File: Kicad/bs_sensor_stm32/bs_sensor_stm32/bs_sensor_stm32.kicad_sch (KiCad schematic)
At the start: 4 parts, among them U1 NRF24L01_Breakout

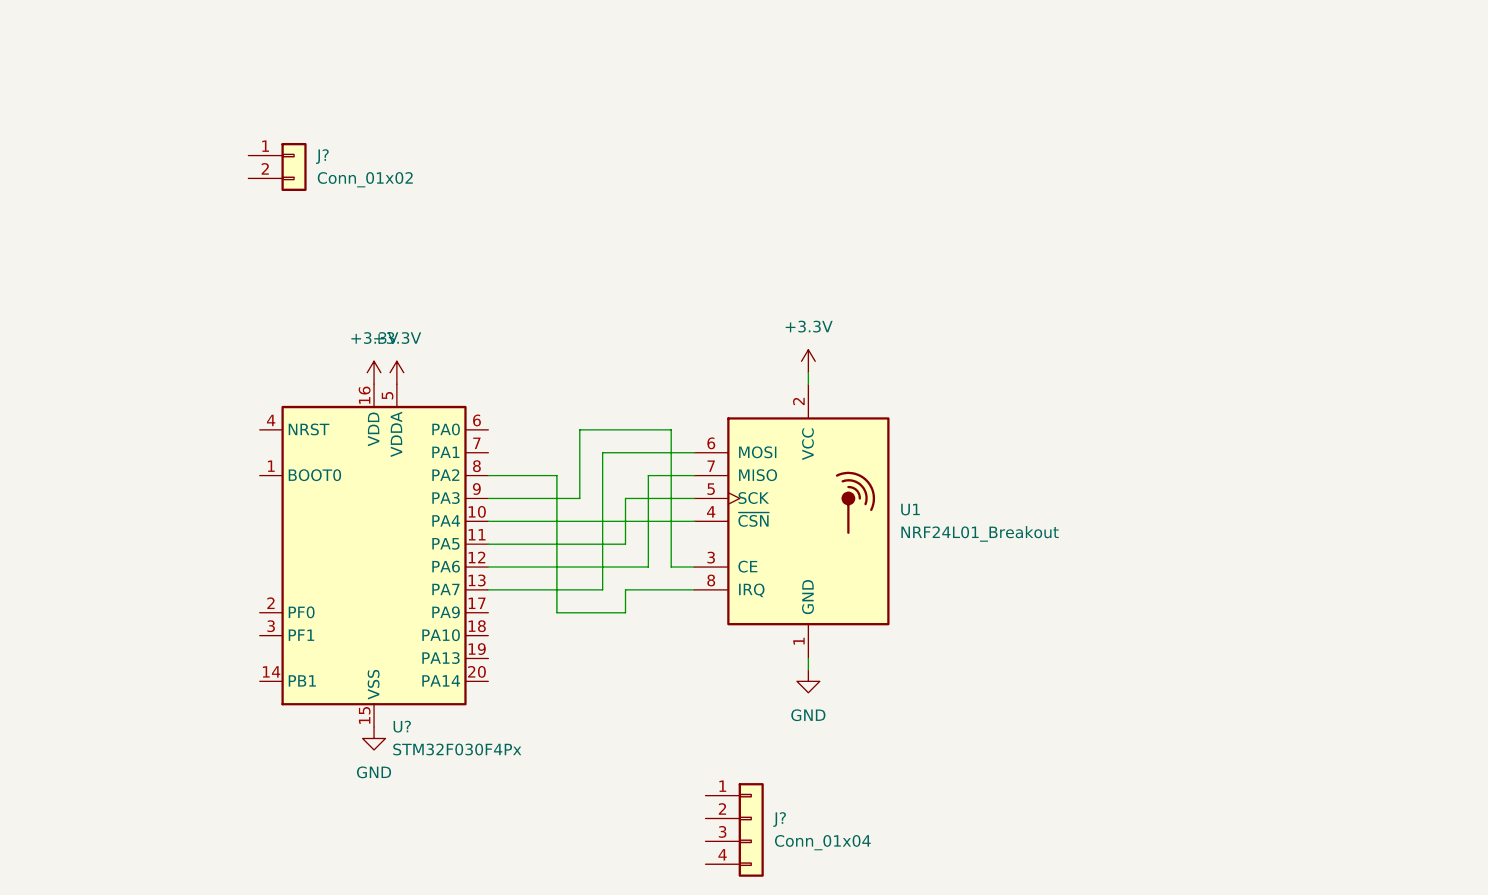
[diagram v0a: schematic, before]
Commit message: 01.03.2022
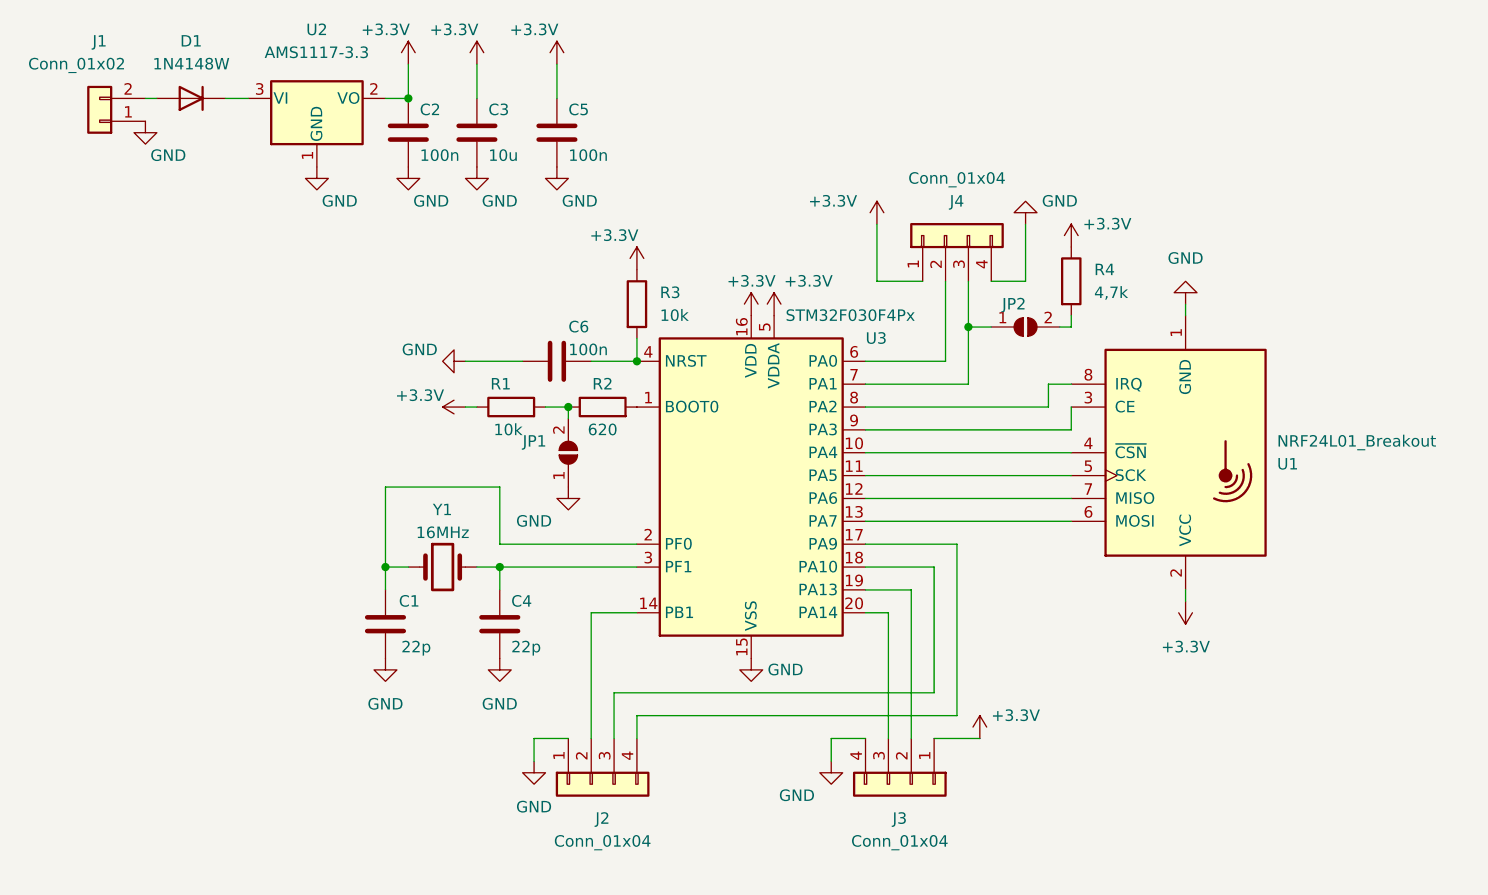
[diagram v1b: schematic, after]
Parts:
- added C1, C4: 22p, Capacitor_SMD:C_0805_2012Metric, symbol Device:C
- added C2, C5, C6: 100n, Capacitor_SMD:C_0805_2012Metric, symbol Device:C
- added C3: 10u, Capacitor_SMD:C_0805_2012Metric, symbol Device:C
- added D1: 1N4148W, Diode_SMD:D_SOD-123, symbol Diode:1N4148W
- added J2, J4: Conn_01x04, Connector_PinHeader_2.54mm:PinHeader_1x04_P2.54mm_Vertical, symbol Connector_Generic:Conn_01x04
- added JP1, JP2: SolderJumper_2_Open, Jumper:SolderJumper-2_P1.3mm_Open_RoundedPad1.0x1.5mm, symbol Jumper:SolderJumper_2_Open
- added R1, R3: 10k, Resistor_SMD:R_0805_2012Metric, symbol Device:R
- added R2: 620, Resistor_SMD:R_0603_1608Metric, symbol Device:R
- added R4: 4,7k, Resistor_SMD:R_0805_2012Metric, symbol Device:R
- added U2: AMS1117-3.3, Package_TO_SOT_SMD:SOT-223-3_TabPin2, symbol Regulator_Linear:AMS1117-3.3
- added Y1: 16MHz, Crystal:Crystal_HC49-U_Vertical, symbol Device:Crystal
- J1: renamed from J?; footprint (none) -> Connector_PinHeader_2.54mm:PinHeader_1x02_P2.54mm_Vertical
- J3: renamed from J?; footprint (none) -> Connector_PinHeader_2.54mm:PinHeader_1x04_P2.54mm_Vertical
- gave numbers to parts that had none: 1
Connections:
- net +3V3: now also J3.1 (Pin_1), C2.1, C3.1, C5.1, J4.1 (Pin_1), R1.1, R3.1, R4.1, U2.2 (VO)
- net GND: now also J1.1 (Pin_1), J3.4 (Pin_4), C1.1, C2.2, C3.2, C4.2, C5.2, C6.2, J2.1 (Pin_1), J4.4 (Pin_4), JP1.1 (A), U2.1 (GND)
- net at U3.1 (BOOT0): now also R2.2
- net at U3.14 (PB1): now also J2.2 (Pin_2)
- net at U3.17 (PA9): now also J2.4 (Pin_4)
- net at U3.18 (PA10): now also J2.3 (Pin_3)
- net at U3.19 (PA13): now also J3.2 (Pin_2)
- net at U3.2 (PF0): now also C1.2, Y1.1
- net at U3.20 (PA14): now also J3.3 (Pin_3)
- net at U3.3 (PF1): now also C4.1, Y1.2
- net at U3.4 (NRST): now also C6.1, R3.2
- net at U3.6 (PA0): now also J4.2 (Pin_2)
- net at U3.7 (PA1): now also J4.3 (Pin_3), JP2.1 (A)
- net at J1.2 (Pin_2): now also D1.2 (A)
- new net: JP2.2 (B), R4.2
- new net: JP1.2 (B), R1.2, R2.1
- new net: D1.1 (K), U2.3 (VI)
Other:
- moved on the sheet: J1, J3, U1, U3

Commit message: 05.03.2022
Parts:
- JP1, JP2: footprint Jumper:SolderJumper-2_P1.3mm_Open_RoundedPad1.0x1.5mm -> Jumper:SolderJumper-2_P1.3mm_Open_TrianglePad1.0x1.5mm
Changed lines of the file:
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@@
       (effects (font (size 1.27 1.27)) hide)
     )
-    (property "Footprint" "Jumper:SolderJumper-2_P1.3mm_Open_RoundedPad1.0x1.5mm" (id 2) (at 139.7 62.23 0)
+    (property "Footprint" "Jumper:SolderJumper-2_P1.3mm_Open_TrianglePad1.0x1.5mm" (id 2) (at 139.7 62.23 0)
       (effects (font (size 1.27 1.27)) hide)
     )
@@
       (effects (font (size 1.27 1.27)) (justify right) hide)
     )
-    (property "Footprint" "Jumper:SolderJumper-2_P1.3mm_Open_RoundedPad1.0x1.5mm" (id 2) (at 88.9 76.2 0)
+    (property "Footprint" "Jumper:SolderJumper-2_P1.3mm_Open_TrianglePad1.0x1.5mm" (id 2) (at 88.9 76.2 0)
       (effects (font (size 1.27 1.27)) hide)
     )
@@
     )
     (path "/ab3124e5-ab45-4ab0-95d1-6c14bd4e9f92"
-      (reference "JP1") (unit 1) (value "SolderJumper_2_Open") (footprint "Jumper:SolderJumper-2_P1.3mm_Open_RoundedPad1.0x1.5mm")
+      (reference "JP1") (unit 1) (value "SolderJumper_2_Open") (footprint "Jumper:SolderJumper-2_P1.3mm_Open_TrianglePad1.0x1.5mm")
     )
     (path "/31bb1625-b0b2-415a-9b3a-13977a6c8055"
-      (reference "JP2") (unit 1) (value "SolderJumper_2_Open") (footprint "Jumper:SolderJumper-2_P1.3mm_Open_RoundedPad1.0x1.5mm")
+      (reference "JP2") (unit 1) (value "SolderJumper_2_Open") (footprint "Jumper:SolderJumper-2_P1.3mm_Open_TrianglePad1.0x1.5mm")
     )
     (path "/a89d2b6c-f370-4c87-af3a-312fe183f96e"
